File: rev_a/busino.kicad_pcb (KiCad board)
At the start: 2 copper layers, 100 x 100 mm, 56 parts, among them J1 TERMINATE_JUMPER, SW1 2_LEAD_PUSH_BUTTON, U1 LM2940CT-5.0, U2 MCP2562, U3 LM1117T-3.3, U4 74x06, U5 ATMEGA324_DIP40, X1 16MHz

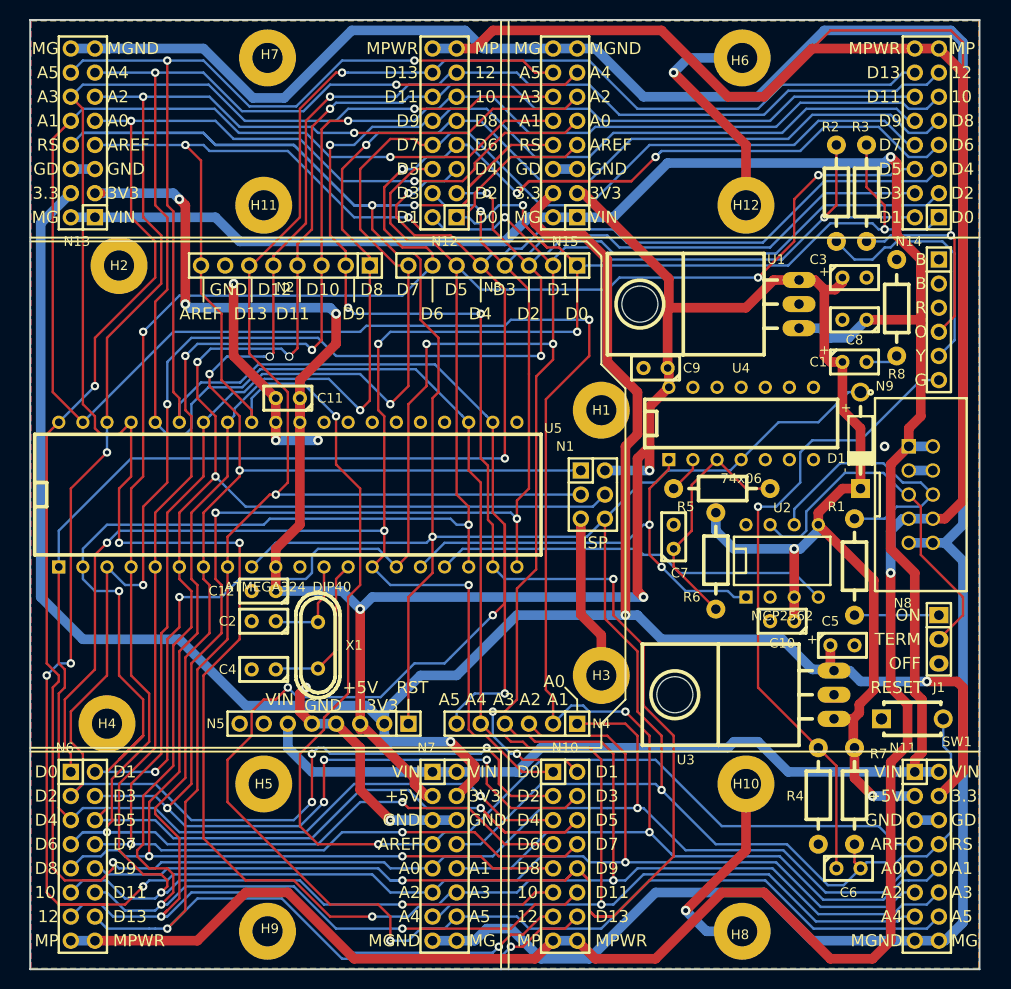
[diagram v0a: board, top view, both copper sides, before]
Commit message: Rev. A of the Busino board layout is in pretty good shape.
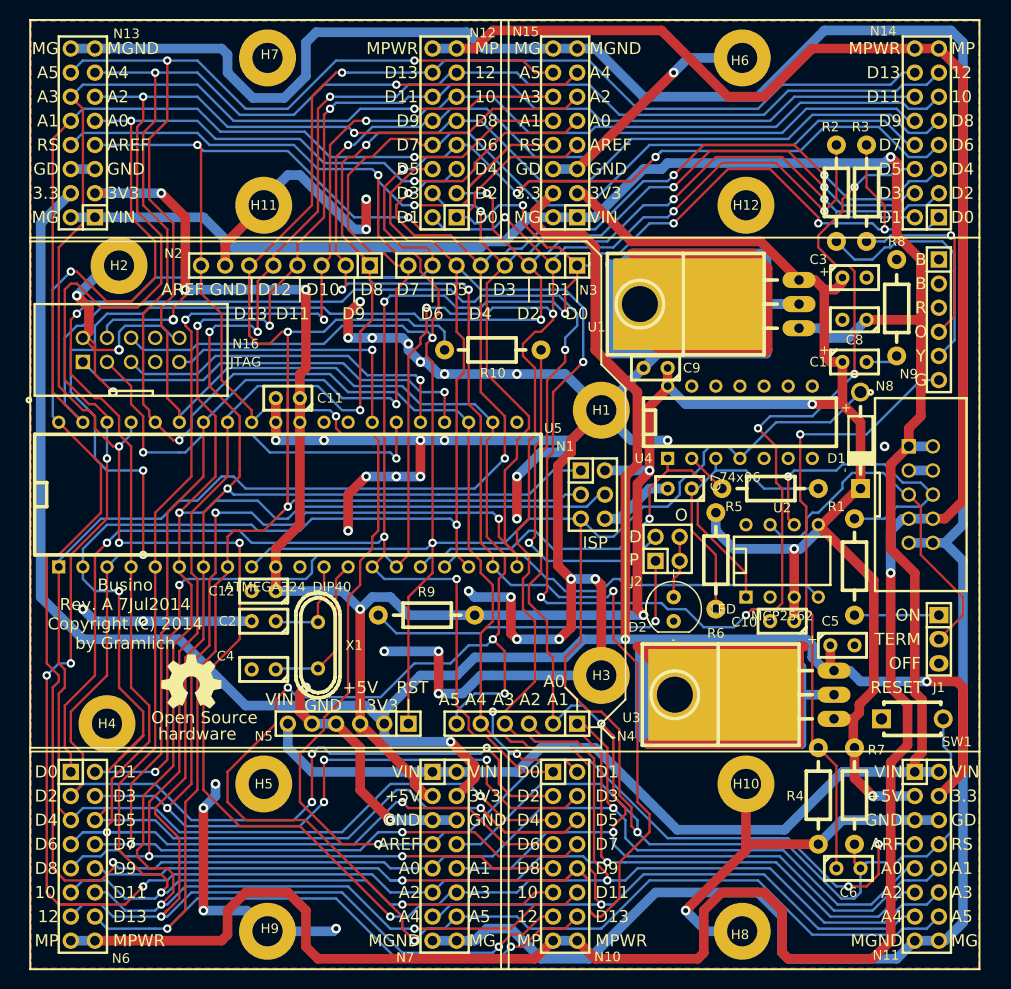
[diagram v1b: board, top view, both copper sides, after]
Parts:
- added D2: LED, Busino_Rev_A:T1_LED, F.Cu at (94.0, 88.3)
- added J2: LED_JUMPER, Busino_Rev_A:Pin_Header_Straight_2x02, F.Cu at (93.3, 81.9)
- added N16: AVR_JTAG_CONNECTOR, Busino_Rev_A:Pin_Header_Straight_2x05_Shrouded, F.Cu at (36.8, 61.0)
- added R10: R_VERT, Busino_Rev_A:Resistor_Horizontal__400, F.Cu at (74.9, 61.0)
- added R9: R_VERT, Busino_Rev_A:Resistor_Horizontal__400, F.Cu at (67.9, 88.9)
- added X2: OSHW_LOGO, Busino_Rev_A:OSHW_LOGO_250mil, F.Cu at (43.2, 95.9)
- N5: footprint Busino_Rev_A:Pin_Header_Straight_1x08 -> Busino_Rev_A:Pin_Header_Straight_1x06
- moved C7 5.12 mm to (94.6, 75.6), turned to 180 degrees
- moved R5 5.08 mm to (104.1, 75.6)
- moved N5 2.54 mm to (59.7, 100.3)
- moved U4 0.18 mm to (101.0, 68.6)
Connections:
- J1 pad 3: Net-(J1-Pad3) -> (no net)
- N1 pad 5: GND -> /Arduino Shield/~RESET
- N1 pad 6: /Arduino Shield/~RESET -> GND
- N9 pad 2: Net-(N9-Pad2) -> (no net)
- N9 pad 3: Net-(N9-Pad3) -> (no net)
- U5 pad 21: Net-(U5-Pad21) -> (no net)
- U5 pad 28: Net-(U5-Pad28) -> (no net)
- U5 pad 29: Net-(U5-Pad29) -> (no net)
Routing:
- net GND: track 124.8 -> 641.1 mm, vias 7 -> 42
- net /Arduino Shield/D5: track 257.8 -> 338.5 mm, vias 5 -> 9
- net /Arduino Shield/MPWR: track 333.5 -> 269.8 mm
- net Net-(N16-Pad1): track 0.00 -> 44.1 mm, vias 0 -> 1
- net Net-(N16-Pad3): track 0.00 -> 43.4 mm, vias 0 -> 2
- net Net-(N16-Pad5): track 0.00 -> 37.3 mm, vias 0 -> 1
- net Net-(J2-Pad1): track 0.00 -> 36.9 mm, vias 0 -> 1
- net /Arduino Shield/D13: track 255.8 -> 292.3 mm, vias 4 -> 5
- net Net-(J2-Pad2): track 0.00 -> 36.0 mm, vias 0 -> 1
- net Net-(N16-Pad9): track 0.00 -> 28.5 mm, vias 0 -> 1
- net /Arduino Shield/D6: track 243.7 -> 262.8 mm
- net /Arduino Shield/D2: track 231.2 -> 245.7 mm, vias 7 -> 9
- net /Arduino Shield/~RESET: track 344.9 -> 358.1 mm, vias 4 -> 5
- net +5V: track 305.5 -> 318.5 mm, vias 8 -> 10
- net /Arduino Shield/A0: track 256.9 -> 268.6 mm
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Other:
- board outline removed
- board text added: "Busino Rev. A 7Jul2014 Copyright (c) 2014 by Gramlich"
- board text added: "D"
- board text added: "JTAG"
- board text added: "Open Source"
- board text added: "P"
- board text added: "hardware"
